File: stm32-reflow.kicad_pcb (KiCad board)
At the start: 4 copper layers, 64.5 x 59.5 mm, 52 parts, among them J1 TC2030, J10 63824-1, J11 63824-1, J12 63824-1, J2 Conn_01x04_Male, J3 Conn_01x03_Male, J4 Screw_Terminal_01x02, J5 Screw_Terminal_01x02, J6 Conn_02x08_Odd_Even, J7 63824-1, J8 63824-1, J9 63824-1, Q1 2N7002, Q10 2N7002, Q11 2N7002, Q2 2N7002, Q3 2N7002, Q4 2N7002, Q5 2N7002, Q6 2N7002, Q7 2N7002, Q8 2N7002, Q9 2N7002, U1 STM32F051R4Tx, U2 MAX31855KASA, U3 MAX31855KASA, Y1 8MHz

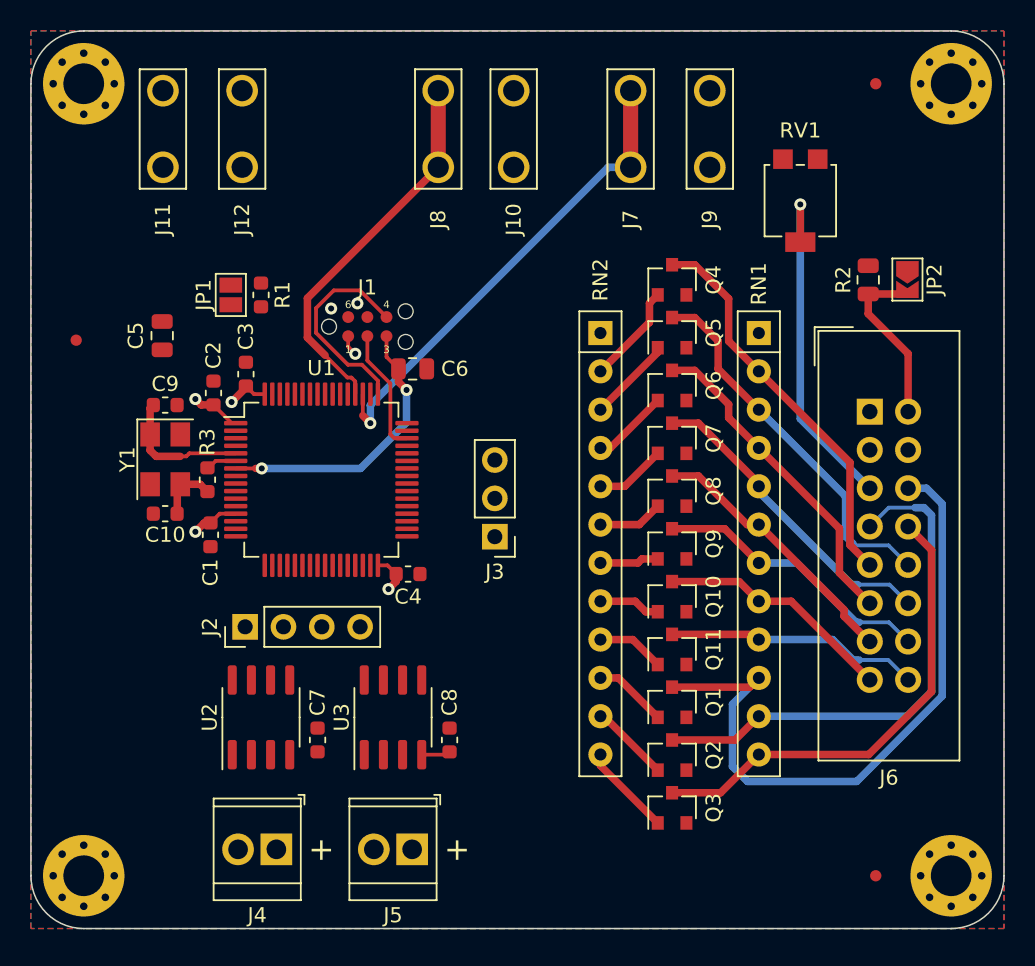
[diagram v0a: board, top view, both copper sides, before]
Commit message: finalized routing and circuit schematic (so far)
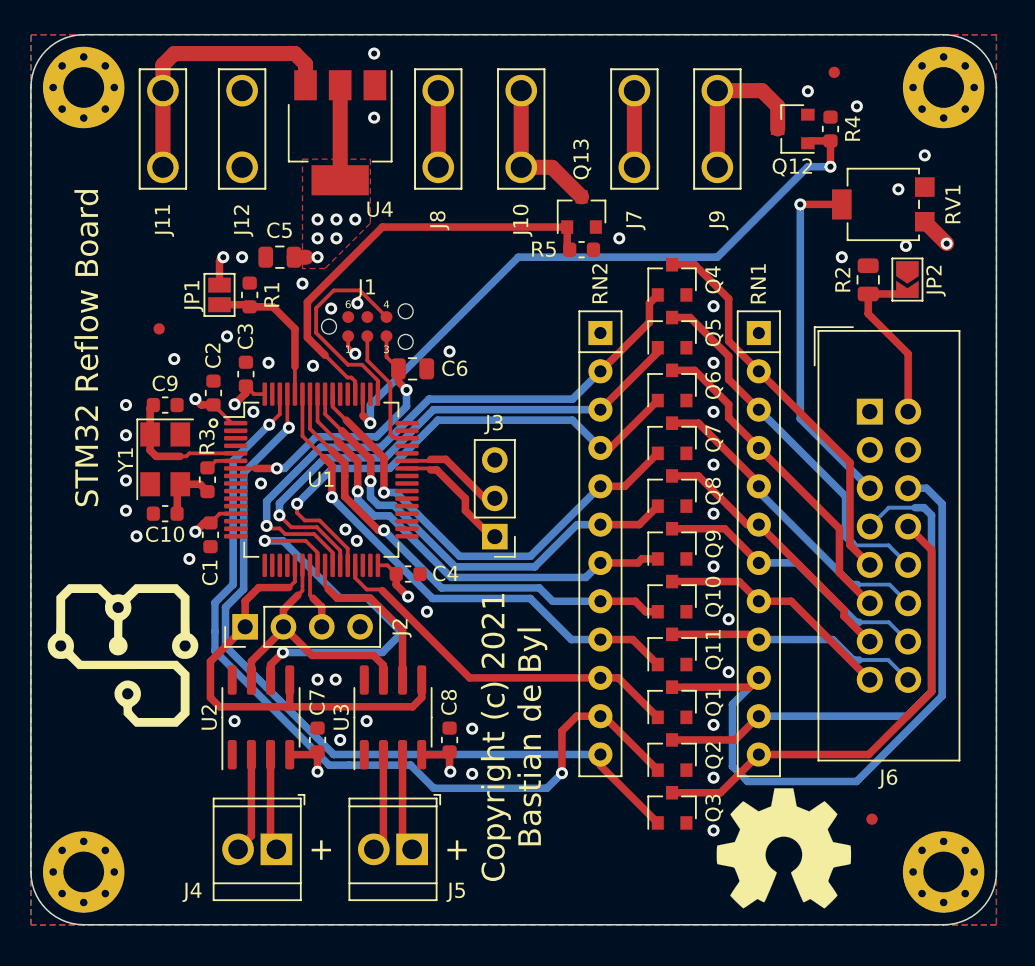
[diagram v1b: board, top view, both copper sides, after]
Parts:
- added G***: LOGO, Personal:db_logo_10mm, F.Cu at (117.6, 115.4)
- added G***: LOGO, Personal:db_logo, B.Cu at (122.8, 91.6)
- added Q12: 2N7002, Package_TO_SOT_SMD:SOT-23, F.Cu at (162.0, 80.5)
- added Q13: 2N7002, Package_TO_SOT_SMD:SOT-23, F.Cu at (148.0, 86.0)
- added R4: 10k, Resistor_SMD:R_0603_1608Metric, F.Cu at (164.5, 80.5)
- added R5: 10k, Resistor_SMD:R_0603_1608Metric, F.Cu at (148.0, 88.5)
- added REF**: OSHW-Symbol_8.9x8mm_SilkScreen, Symbol:OSHW-Symbol_8.9x8mm_SilkScreen, F.Cu at (161.4, 128.2)
- added U4: LM1117-3.3, Package_TO_SOT_SMD:SOT-223-3_TabPin2, F.Cu at (132.0, 80.8)
- moved C5 9.37 mm to (128.0, 89.0), turned to 180 degrees
- moved FID3 5.55 mm to (120.0, 93.8)
- moved RV1 5.51 mm to (168.0, 85.5), turned to -90 degrees
- moved FID2 3.76 mm to (167.2, 126.2)
- moved FID1 2.85 mm to (164.8, 76.8)
- moved JP1 0.75 mm to (124.0, 91.5)
- moved R1 0.75 mm to (126.0, 91.5), turned to 90 degrees
- moved H1 0.56 mm to (172.0, 77.8)
- moved H3 0.56 mm to (172.0, 129.8)
- moved J10 0.50 mm to (144.0, 80.5)
- moved J9 0.50 mm to (157.0, 80.5)
- moved H2 0.25 mm to (115.0, 129.8)
- moved H4 0.25 mm to (115.0, 77.8)
- moved J7 0.25 mm to (151.5, 80.5)
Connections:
- J10 pad 1: GND -> Net-(J10-Pad1)
- J10 pad 2: GND -> Net-(J10-Pad1)
- J7 pad 1: /Reflow MCU/R1E -> +5V
- J7 pad 2: /Reflow MCU/R1E -> +5V
- J8 pad 1: /Reflow MCU/R2E -> +5V
- J8 pad 2: /Reflow MCU/R2E -> +5V
- J9 pad 1: GND -> Net-(J9-Pad1)
- J9 pad 2: GND -> Net-(J9-Pad1)
- U3 pad 6: /Reflow MCU/CS0 -> /Reflow MCU/CS1
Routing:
- net /Reflow Level Shifting/R/~{W}: track 5.28 -> 57.0 mm, vias 0 -> 2
- net /Reflow Level Shifting/E: track 6.11 -> 52.4 mm, vias 0 -> 1
- net /Reflow Level Shifting/DB0: track 6.64 -> 39.9 mm, vias 0 -> 1
- net /Reflow Level Shifting/DB1: track 5.68 -> 36.3 mm, vias 0 -> 1
- net +5V: track 0.00 -> 30.5 mm, vias 0 -> 1
- net /Reflow MCU/SCK: track 0.00 -> 29.7 mm
- net /Reflow Level Shifting/DB7: track 4.49 -> 33.9 mm, vias 0 -> 1
- net /Reflow Level Shifting/DB2: track 5.10 -> 34.3 mm, vias 0 -> 1
- net /Reflow Level Shifting/DB6: track 4.09 -> 31.7 mm, vias 0 -> 1
- net /Reflow MCU/CS0: track 0.00 -> 26.8 mm, vias 0 -> 2
- net /Reflow Level Shifting/DB5: track 3.91 -> 30.6 mm, vias 0 -> 1
- net /Reflow Level Shifting/DB4: track 4.31 -> 30.7 mm, vias 0 -> 1
- net /Reflow Level Shifting/DB3: track 4.71 -> 30.7 mm, vias 0 -> 1
- net /Reflow Level Shifting/RS: track 4.88 -> 24.7 mm
- net /Reflow MCU/MISO: track 0.00 -> 17.7 mm
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- added copper zone on F.Cu, net +3V3
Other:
- board size 64.5 x 59.5 mm -> 64 x 59 mm
- board text added: "Copyright (c) 2021 Bastian de Byl"
- board text added: "STM32 Reflow Board"
- board text added: "STM32 Reflow Board Designed by Bastian de Byl"
